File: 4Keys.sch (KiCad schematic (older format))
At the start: 29 parts, among them J1 OLED1, J2 OLED2, SW1 SW_Reset, U1 ATmega32U4-AU, Y1 16MHz

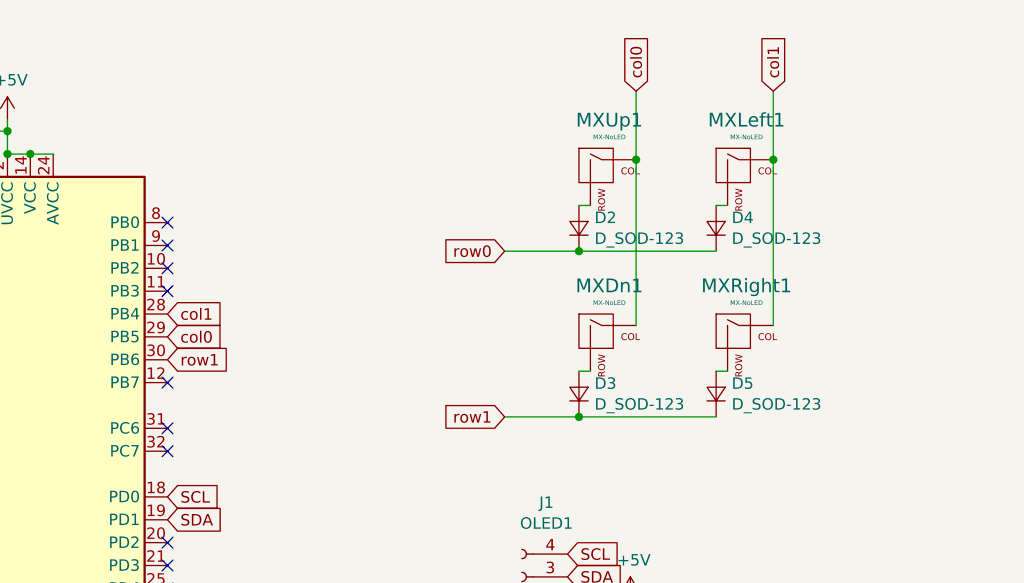
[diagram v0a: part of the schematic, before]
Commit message: UPDATE PCB
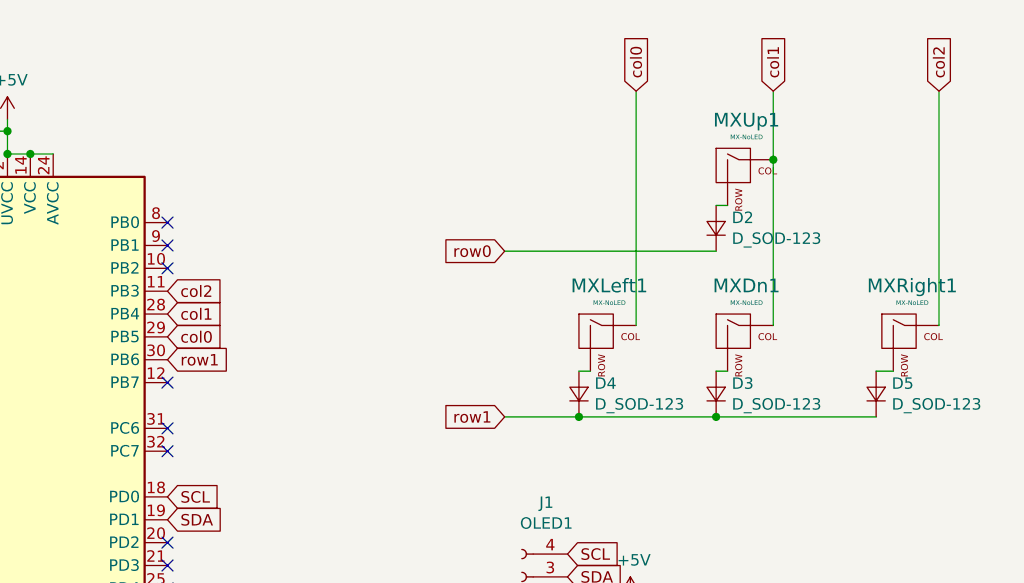
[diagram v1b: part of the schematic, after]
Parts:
- J1, J2: footprint Connector_PinHeader_2.54mm:PinHeader_1x04_P2.54mm_Vertical -> Connector_JST:JST_EH_S4B-EH_1x04_P2.50mm_Horizontal
- USB1: footprint (none) -> mullet:HRO-TYPE-C-31-M-12-HandSoldering
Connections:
- net col0: now also MXLeft1.1 (COL); no longer MXDn1.1 (COL), MXUp1.1 (COL)
- net col1: now also MXDn1.1 (COL), MXUp1.1 (COL); no longer MXLeft1.1 (COL), MXRight1.1 (COL)
- net row0: no longer D4.1 (K)
- net row1: now also D4.1 (K)
- net col2: now reaches U1.11 (PB3)
- net col2: now also MXRight1.1 (COL)
- no-connect marks 22 -> 21
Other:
- moved on the sheet: D2, D3, D4, D5, MXDn1, MXLeft1, MXRight1, MXUp1
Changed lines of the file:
@@
 F 0 "USB1" H 1750 7500 60  0000 C CNN
 F 1 "mullet-pcb-rescue_HRO-TYPE-C-31-M-12-Type-C" H 1950 6000 60  0000 C CNN
-F 2 "" H 1950 6850 60  0001 C CNN
+F 2 "mullet:HRO-TYPE-C-31-M-12-HandSoldering" H 1950 6850 60  0001 C CNN
 F 3 "" H 1950 6850 60  0001 C CNN
 	1    1950 6850
@@
 	2125 7500 2125 7400
 $Comp
-L MX_Alps_Hybrid:MX-NoLED MXUp1
-U 1 1 5E7BC528
-P 4600 1375
-F 0 "MXUp1" H 4633 1598 60  0000 C CNN
-F 1 "MX-NoLED" H 4633 1524 20  0000 C CNN
-F 2 "MX_Alps_Hybrid:MX-1U-NoLED" H 3975 1350 60  0001 C CNN
-F 3 "" H 3975 1350 60  0001 C CNN
-	1    4600 1375
-	1    0    0    -1
-$EndComp
-$Comp
 L Device:D_Small D2
 U 1 1 5E7BCC47
-P 4500 1625
-F 0 "D2" V 4546 1557 50  0000 R CNN
-F 1 "D_SOD-123" V 4455 1557 50  0000 R CNN
-F 2 "Diode_SMD:D_0805_2012Metric" V 4500 1625 50  0001 C CNN
-F 3 "~" V 4500 1625 50  0001 C CNN
-	1    4500 1625
-	0    -1   -1   0
-$EndComp
-Wire Wire Line
-	4500 1525 4550 1525
-$Comp
-L MX_Alps_Hybrid:MX-NoLED MXLeft1
-U 1 1 5E7BF41E
-P 5200 1375
-F 0 "MXLeft1" H 5233 1598 60  0000 C CNN
-F 1 "MX-NoLED" H 5233 1524 20  0000 C CNN
-F 2 "MX_Alps_Hybrid:MX-1U-NoLED" H 4575 1350 60  0001 C CNN
-F 3 "" H 4575 1350 60  0001 C CNN
-	1    5200 1375
-	1    0    0    -1
-$EndComp
-$Comp
-L Device:D_Small D4
-U 1 1 5E7BF7DA
 P 5100 1625
-F 0 "D4" V 5146 1557 50  0000 R CNN
+F 0 "D2" V 5146 1557 50  0000 R CNN
 F 1 "D_SOD-123" V 5055 1557 50  0000 R CNN
 F 2 "Diode_SMD:D_0805_2012Metric" V 5100 1625 50  0001 C CNN
@@
 $EndComp
 $Comp
-L MX_Alps_Hybrid:MX-NoLED MXDn1
-U 1 1 5E7C1351
+L MX_Alps_Hybrid:MX-NoLED MXLeft1
+U 1 1 5E7BF41E
 P 4600 2100
-F 0 "MXDn1" H 4633 2323 60  0000 C CNN
+F 0 "MXLeft1" H 4633 2323 60  0000 C CNN
 F 1 "MX-NoLED" H 4633 2249 20  0000 C CNN
 F 2 "MX_Alps_Hybrid:MX-1U-NoLED" H 3975 2075 60  0001 C CNN
@@
 $EndComp
 $Comp
-L Device:D_Small D3
-U 1 1 5E7C17AD
+L Device:D_Small D4
+U 1 1 5E7BF7DA
 P 4500 2350
-F 0 "D3" V 4546 2282 50  0000 R CNN
+F 0 "D4" V 4546 2282 50  0000 R CNN
 F 1 "D_SOD-123" V 4455 2282 50  0000 R CNN
 F 2 "Diode_SMD:D_0805_2012Metric" V 4500 2350 50  0001 C CNN
@@
 	0    -1   -1   0
 $EndComp
-Wire Wire Line
-	4500 2250 4550 2250
-$Comp
-L MX_Alps_Hybrid:MX-NoLED MXRight1
-U 1 1 5E7C36BC
+$Comp
+L MX_Alps_Hybrid:MX-NoLED MXDn1
+U 1 1 5E7C1351
 P 5200 2100
-F 0 "MXRight1" H 5233 2323 60  0000 C CNN
+F 0 "MXDn1" H 5233 2323 60  0000 C CNN
 F 1 "MX-NoLED" H 5233 2249 20  0000 C CNN
 F 2 "MX_Alps_Hybrid:MX-1U-NoLED" H 4575 2075 60  0001 C CNN
@@
 $EndComp
 $Comp
-L Device:D_Small D5
-U 1 1 5E7C3AB9
+L Device:D_Small D3
+U 1 1 5E7C17AD
 P 5100 2350
-F 0 "D5" V 5146 2282 50  0000 R CNN
+F 0 "D3" V 5146 2282 50  0000 R CNN
 F 1 "D_SOD-123" V 5055 2282 50  0000 R CNN
 F 2 "Diode_SMD:D_0805_2012Metric" V 5100 2350 50  0001 C CNN
@@
 	0    -1   -1   0
 $EndComp
+$Comp
+L MX_Alps_Hybrid:MX-NoLED MXRight1
+U 1 1 5E7C36BC
+P 5925 2100
+F 0 "MXRight1" H 5958 2323 60  0000 C CNN
+F 1 "MX-NoLED" H 5958 2249 20  0000 C CNN
+F 2 "MX_Alps_Hybrid:MX-1U-NoLED" H 5300 2075 60  0001 C CNN
+F 3 "" H 5300 2075 60  0001 C CNN
+	1    5925 2100
+	1    0    0    -1
+$EndComp
+$Comp
+L Device:D_Small D5
+U 1 1 5E7C3AB9
+P 5800 2350
+F 0 "D5" V 5846 2282 50  0000 R CNN
+F 1 "D_SOD-123" V 5755 2282 50  0000 R CNN
+F 2 "Diode_SMD:D_0805_2012Metric" V 5800 2350 50  0001 C CNN
+F 3 "~" V 5800 2350 50  0001 C CNN
+	1    5800 2350
+	0    -1   -1   0
+$EndComp
 Wire Wire Line
 	5100 2250 5150 2250
-Wire Wire Line
-	4750 1325 4750 2050
-Wire Wire Line
-	5350 1325 5350 2050
-Wire Wire Line
-	5100 2450 4500 2450
-Wire Wire Line
-	5100 1725 4500 1725
 Text GLabel 4750 1025 1    50   Input ~ 0
 col0
@@
 Text GLabel 4175 2450 0    50   Input ~ 0
 row1
-Wire Wire Line
-	4500 2450 4175 2450
-Connection ~ 4500 2450
-Wire Wire Line
-	4500 1725 4175 1725
-Connection ~ 4500 1725
-Wire Wire Line
-	4750 1025 4750 1325
-Connection ~ 4750 1325
-Wire Wire Line
-	5350 1325 5350 1025
-Connection ~ 5350 1325
-Wire Wire Line
-	5100 1525 5150 1525
 Text GLabel 2700 2100 2    50   Input ~ 0
 col0
@@
 F 0 "J1" H 4142 2825 50  0000 C CNN
 F 1 "OLED1" H 4142 2916 50  0000 C CNN
-F 2 "Connector_PinHeader_2.54mm:PinHeader_1x04_P2.54mm_Vertical" H 4250 3250 50  0001 C CNN
+F 2 "Connector_JST:JST_EH_S4B-EH_1x04_P2.50mm_Horizontal" H 4250 3250 50  0001 C CNN
 F 3 "~" H 4250 3250 50  0001 C CNN
 	1    4250 3250
@@
 F 0 "J2" H 4142 3500 50  0000 C CNN
 F 1 "OLED2" H 4142 3591 50  0000 C CNN
-F 2 "Connector_PinHeader_2.54mm:PinHeader_1x04_P2.54mm_Vertical" H 4250 3925 50  0001 C CNN
+F 2 "Connector_JST:JST_EH_S4B-EH_1x04_P2.50mm_Horizontal" H 4250 3925 50  0001 C CNN
 F 3 "~" H 4250 3925 50  0001 C CNN
 	1    4250 3925
@@
 NoConn ~ 2700 2500
 NoConn ~ 2700 2300
-NoConn ~ 2700 1900
 NoConn ~ 2700 1800
 NoConn ~ 2700 1700
 NoConn ~ 2700 1600
 NoConn ~ 1500 2200
+$Comp
+L MX_Alps_Hybrid:MX-NoLED MXUp1
+U 1 1 5E7BC528
+P 5200 1375
+F 0 "MXUp1" H 5233 1598 60  0000 C CNN
+F 1 "MX-NoLED" H 5233 1524 20  0000 C CNN
+F 2 "MX_Alps_Hybrid:MX-1U-NoLED" H 4575 1350 60  0001 C CNN
+F 3 "" H 4575 1350 60  0001 C CNN
+	1    5200 1375
+	1    0    0    -1
+$EndComp
+Wire Wire Line
+	4175 2450 4500 2450
+Connection ~ 4500 2450
+Wire Wire Line
+	4500 2450 5100 2450
+Wire Wire Line
+	4500 2250 4550 2250
+Wire Wire Line
+	5100 2450 5800 2450
+Connection ~ 5100 2450
+Wire Wire Line
+	5800 2250 5875 2250
+Text GLabel 6075 1025 1    50   Input ~ 0
+col2
+Wire Wire Line
+	6075 1025 6075 2050
+Wire Wire Line
+	5100 1525 5150 1525
+Wire Wire Line
+	4175 1725 5100 1725
+Wire Wire Line
+	4750 1025 4750 2050
+Wire Wire Line
+	5350 1025 5350 1325
+Wire Wire Line
+	5350 1325 5350 2050
+Connection ~ 5350 1325
+Text GLabel 2700 1900 2    50   Input ~ 0
+col2
 $EndSCHEMATC
